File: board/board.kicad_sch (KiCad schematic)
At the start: 22 parts, among them J1 24pin FPC, 0.5mm, Q1 Si1308EDL

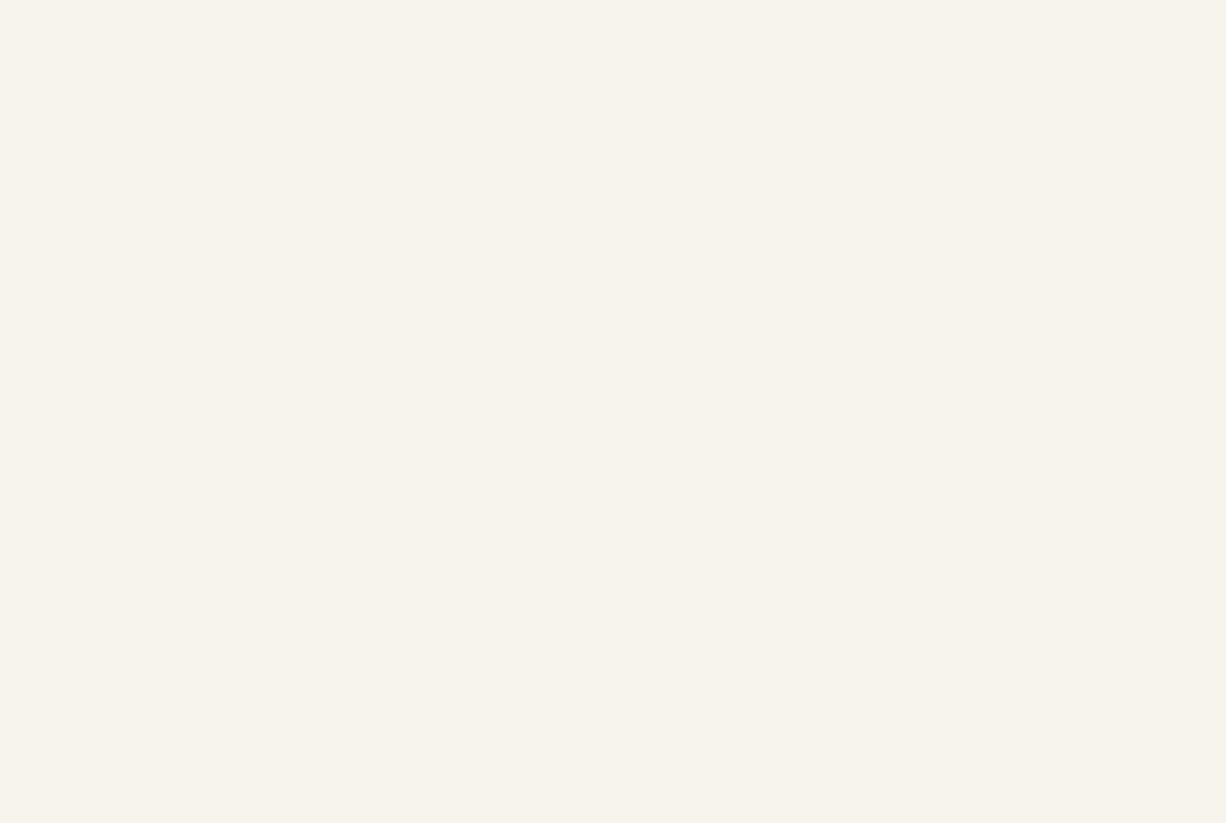
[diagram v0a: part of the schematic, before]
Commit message: Hello Power!
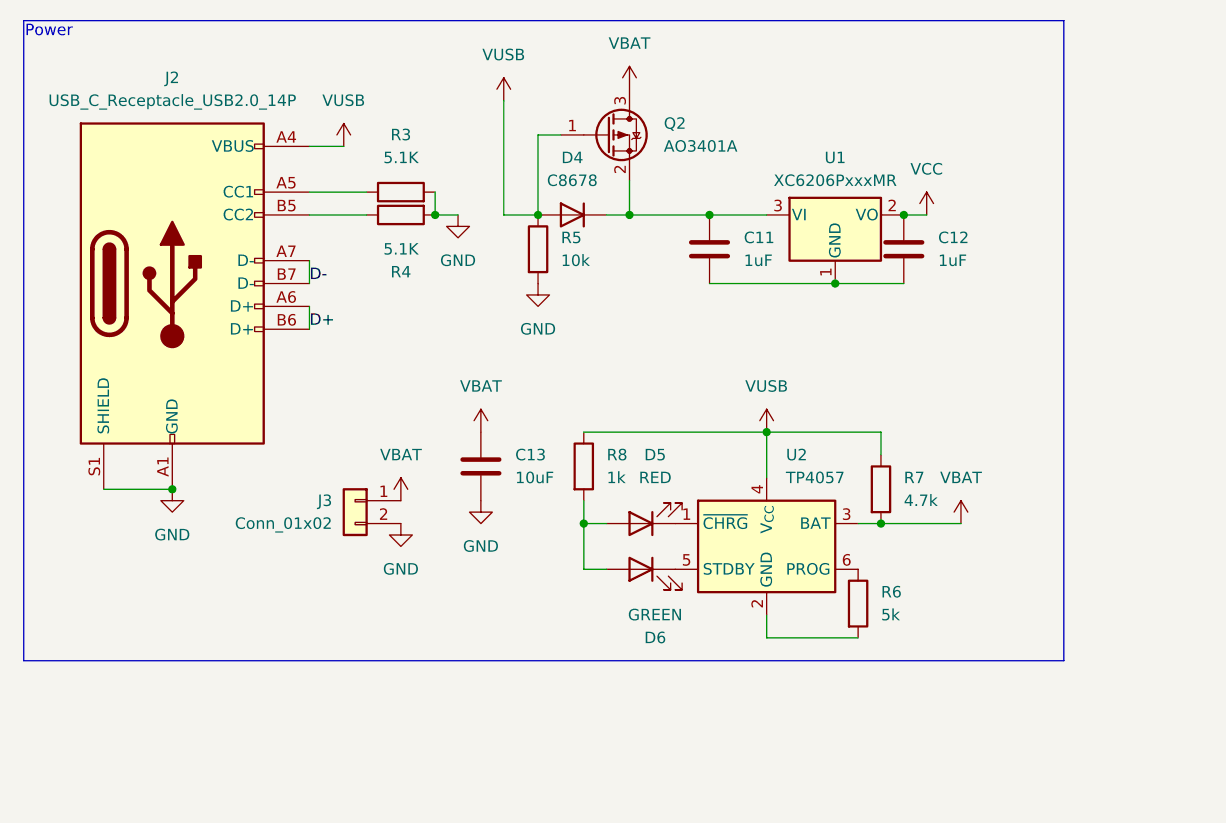
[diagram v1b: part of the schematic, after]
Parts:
- added C11, C12: 1uF, Capacitor_SMD:C_0805_2012Metric_Pad1.18x1.45mm_HandSolder, symbol Device:C
- added C13: 10uF, Capacitor_SMD:C_0805_2012Metric_Pad1.18x1.45mm_HandSolder, symbol Device:C
- added D4: C8678, symbol Device:D
- added D5: RED, symbol Device:LED
- added D6: GREEN, symbol Device:LED
- added J2: USB_C_Receptacle_USB2.0_14P, symbol Connector:USB_C_Receptacle_USB2.0_14P
- added J3: Conn_01x02, symbol Connector_Generic:Conn_01x02
- added Q2: AO3401A, Package_TO_SOT_SMD:SOT-23, symbol Transistor_FET:AO3401A
- added R3, R4: 5.1K, Resistor_SMD:R_0805_2012Metric_Pad1.20x1.40mm_HandSolder, symbol Device:R
- added R5: 10k, Resistor_SMD:R_0805_2012Metric_Pad1.20x1.40mm_HandSolder, symbol Device:R
- added R6: 5k, Resistor_SMD:R_0805_2012Metric_Pad1.20x1.40mm_HandSolder, symbol Device:R
- added R7: 4.7k, Resistor_SMD:R_0805_2012Metric_Pad1.20x1.40mm_HandSolder, symbol Device:R
- added R8: 1k, Resistor_SMD:R_0805_2012Metric_Pad1.20x1.40mm_HandSolder, symbol Device:R
- added U1: XC6206PxxxMR, Package_TO_SOT_SMD:SOT-23-3, symbol Regulator_Linear:XC6206PxxxMR
- added U2: TP4057, Package_TO_SOT_SMD:TSOT-23-6, symbol Battery_Management:TP4057
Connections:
- net GND: now also C13.2, J2.A1 (GND), J2.A12 (GND), J2.B1 (GND), J2.B12 (GND), J2.S1 (SHIELD), J3.2 (Pin_2), R3.2, R4.2, R5.2
- new net: C11.1, D4.1 (K), Q2.2 (S), U1.3 (VI)
- new net: D5.2 (A), D6.2 (A), R8.2
- new net: R6.1, U2.6 (PROG)
- new net: R6.2, U2.2 (GND)
- new net: J2.B5 (CC2), R4.1
- new net: J2.A5 (CC1), R3.1
- new net: D6.1 (K), U2.5 (STDBY)
- new net: C11.2, C12.2, U1.1 (GND)
- new net: D5.1 (K), U2.1 (~{CHRG})
- new net D+: J2.A6 (D+), J2.B6 (D+)
- new net D-: J2.A7 (D-), J2.B7 (D-)
- new net VBAT: C13.1, J3.1 (Pin_1), Q2.3 (D), R7.2, U2.3 (BAT)
- new net VCC: C12.1, U1.2 (VO)
- new net VUSB: D4.2 (A), J2.A4 (VBUS), J2.A9 (VBUS), J2.B4 (VBUS), J2.B9 (VBUS), Q2.1 (G), R5.1, R7.1, R8.1, U2.4 (V_{CC})
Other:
- note added: "Power"
